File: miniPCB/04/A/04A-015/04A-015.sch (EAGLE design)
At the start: 32 parts

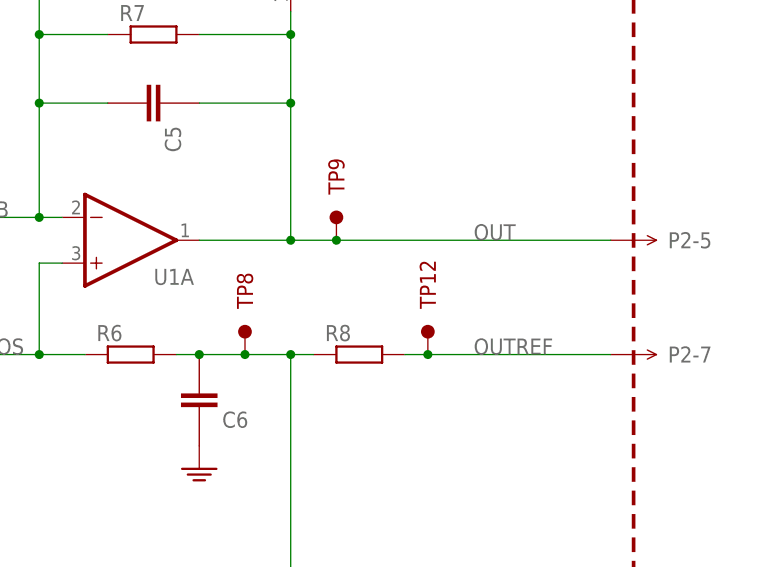
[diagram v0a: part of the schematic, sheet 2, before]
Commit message: NM.03OCT2023
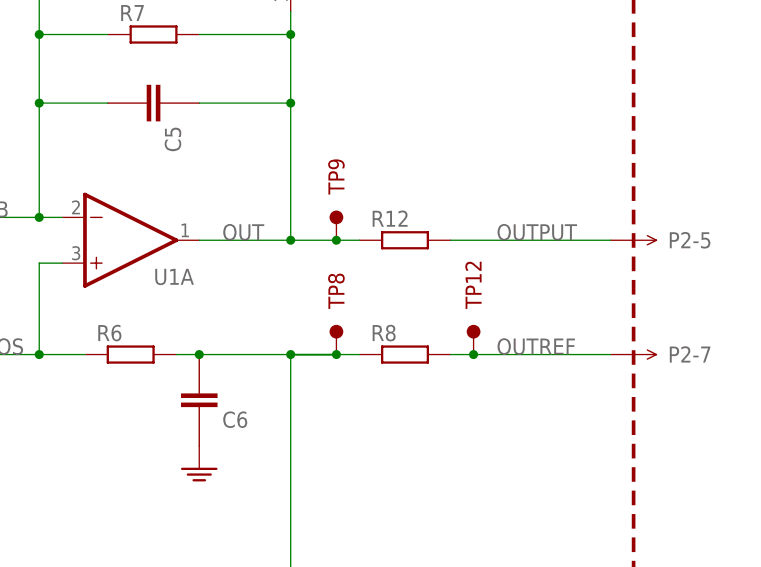
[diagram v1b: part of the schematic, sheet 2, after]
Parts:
- added R12: (no value), minipcb:RESISTOR10MM
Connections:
- new net OUTPUT: P2-5.1, R12.2
- net OUT: now also R12.1; no longer P2-5.1
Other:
- moved on the sheet: R8, TP12, TP8
